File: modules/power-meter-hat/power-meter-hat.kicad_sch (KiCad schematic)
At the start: 25 parts, among them J1 Barrel_Jack_Switch, J2 GPIO, Q1 BC856BDW1, Q2 SI2301CDS, U1 CAT24C256, U2 NCP1117-3.3_SOT223

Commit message: Change jumpers
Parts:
- F1: footprint Fuse:Fuse_1812_4532Metric_Castellated -> Fuse:Fuse_1812_4532Metric

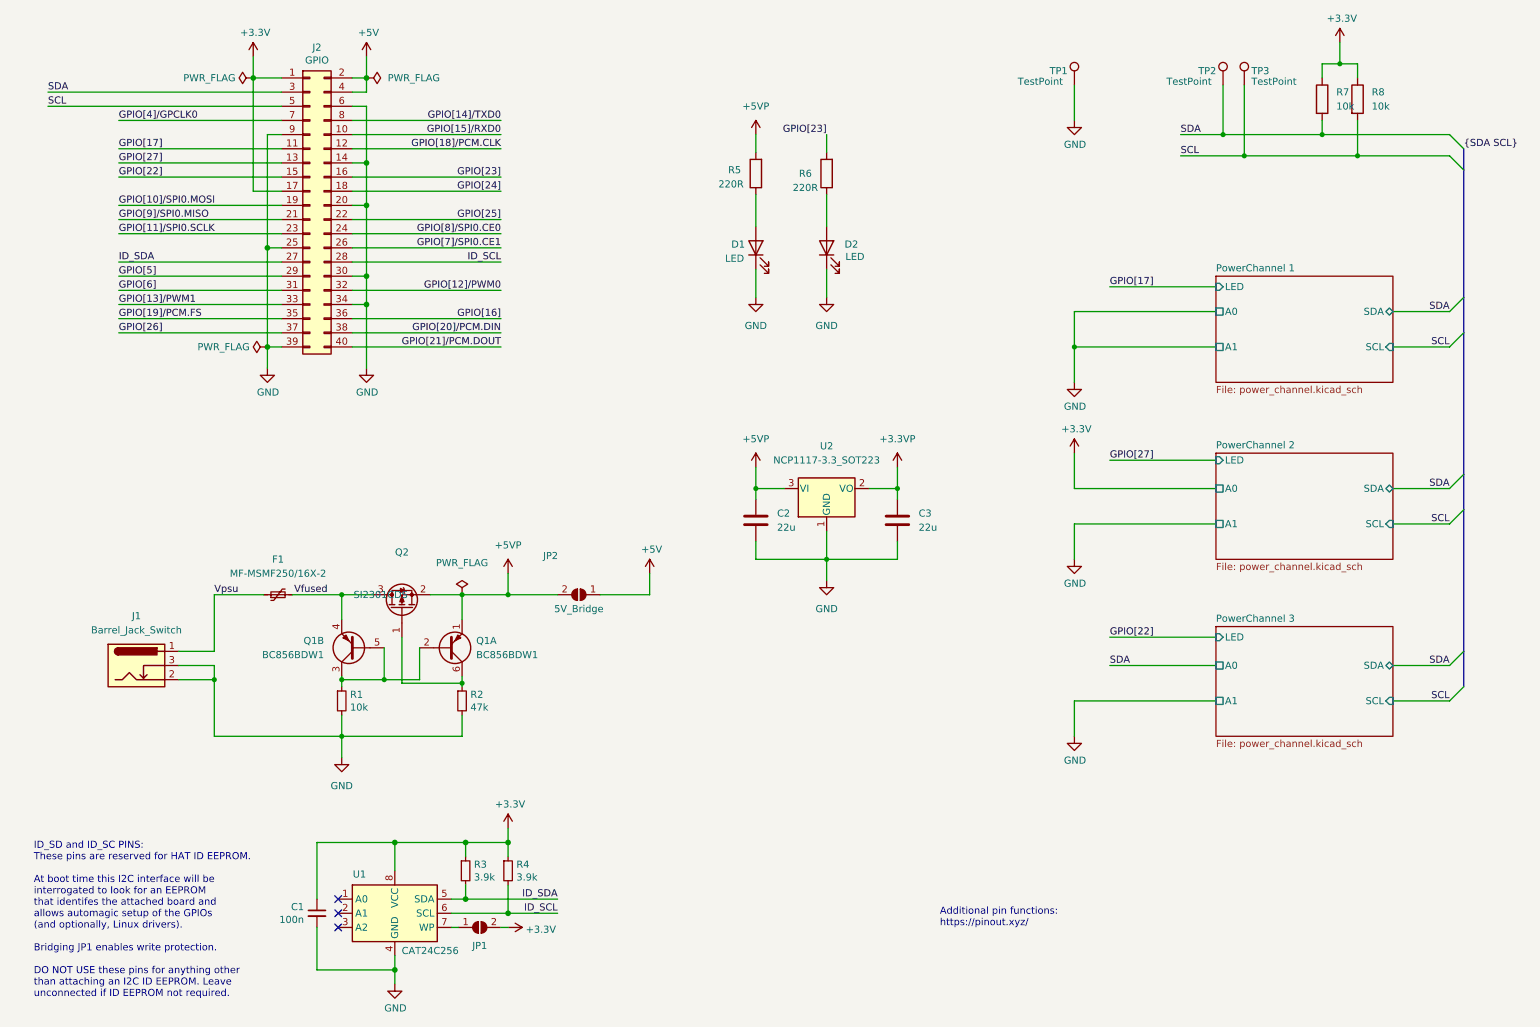
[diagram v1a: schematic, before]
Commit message: Cleanup schematic & PCB
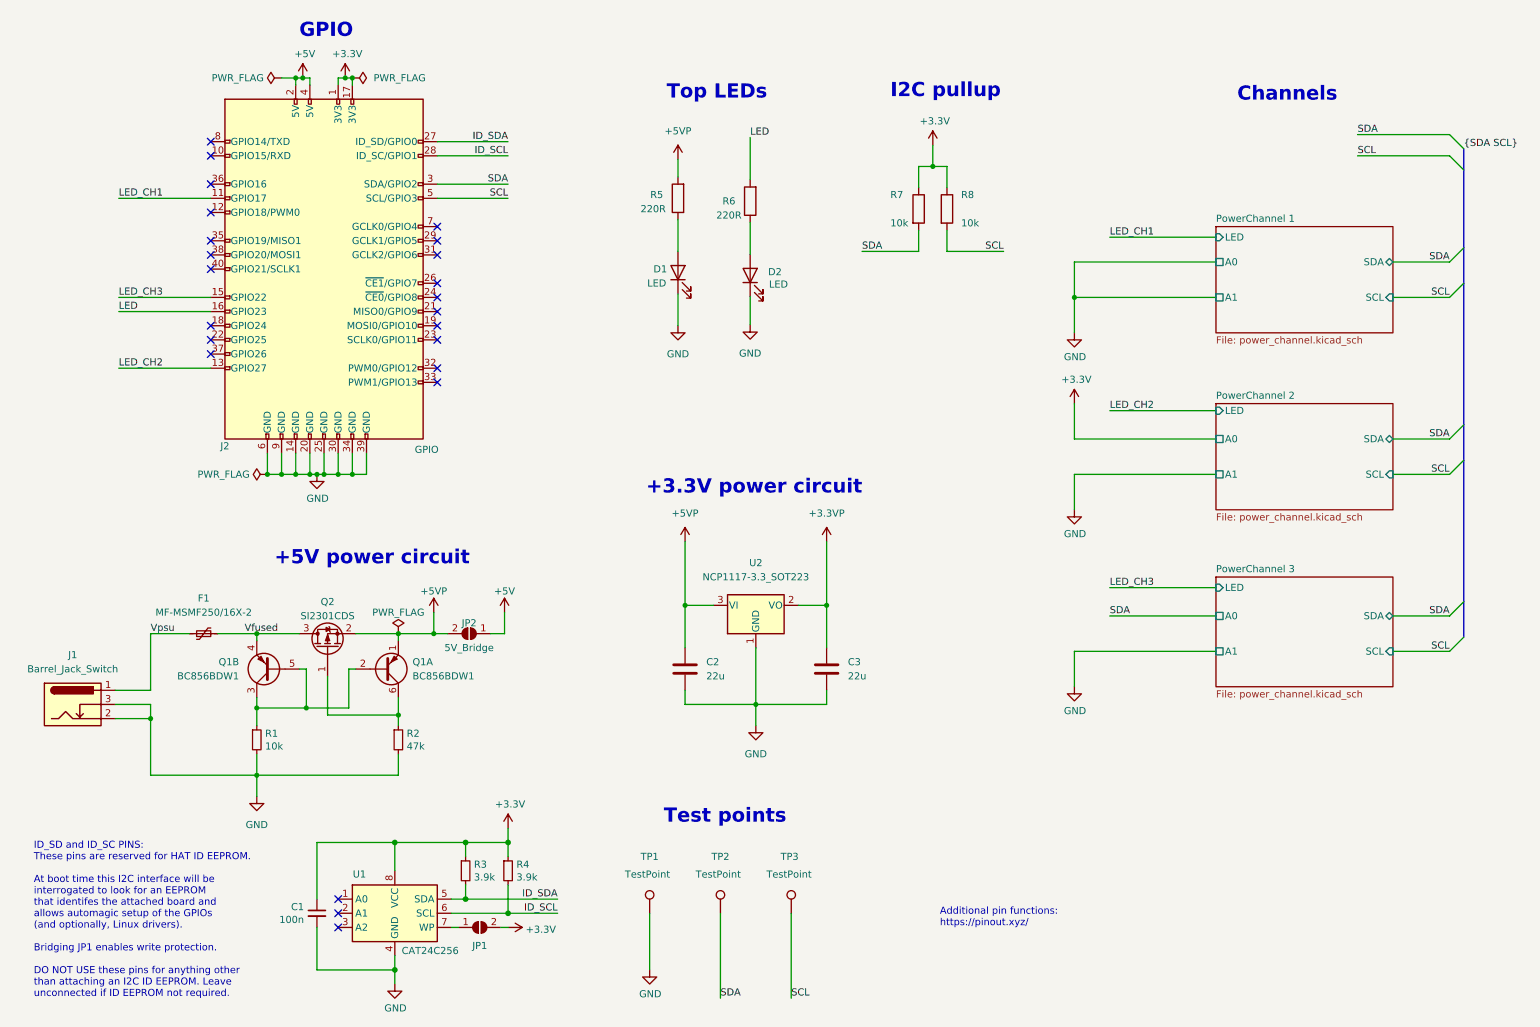
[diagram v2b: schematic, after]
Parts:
- J2: symbol Connector_Generic:Conn_02x20_Odd_Even -> Connector:Raspberry_Pi_2_3
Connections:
- net GPIO[10]/SPI0.MOSI: no longer names the net of J2.19 (MOSI0/GPIO10)
- net GPIO[11]/SPI0.SCLK: no longer names the net of J2.23 (SCLK0/GPIO11)
- net GPIO[12]/PWM0: no longer names the net of J2.32 (PWM0/GPIO12)
- net GPIO[13]/PWM1: no longer names the net of J2.33 (PWM1/GPIO13)
- net GPIO[14]/TXD0: no longer names the net of J2.8 (GPIO14/TXD)
- net GPIO[15]/RXD0: no longer names the net of J2.10 (GPIO15/RXD)
- net GPIO[16]: no longer names the net of J2.36 (GPIO16)
- net GPIO[17] renamed LED_CH1
- net GPIO[18]/PCM.CLK: no longer names the net of J2.12 (GPIO18/PWM0)
- net GPIO[19]/PCM.FS: no longer names the net of J2.35 (GPIO19/MISO1)
- net GPIO[20]/PCM.DIN: no longer names the net of J2.38 (GPIO20/MOSI1)
- net GPIO[21]/PCM.DOUT: no longer names the net of J2.40 (GPIO21/SCLK1)
- net GPIO[22] renamed LED_CH3
- net GPIO[23] renamed LED
- net GPIO[24]: no longer names the net of J2.18 (GPIO24)
- net GPIO[25]: no longer names the net of J2.22 (GPIO25)
- net GPIO[26]: no longer names the net of J2.37 (GPIO26)
- net GPIO[27] renamed LED_CH2
- net GPIO[4]/GPCLK0: no longer names the net of J2.7 (GCLK0/GPIO4)
- net GPIO[5]: no longer names the net of J2.29 (GCLK1/GPIO5)
- net GPIO[6]: no longer names the net of J2.31 (GCLK2/GPIO6)
- net GPIO[7]/SPI0.CE1: no longer names the net of J2.26 (~{CE1}/GPIO7)
- net GPIO[8]/SPI0.CE0: no longer names the net of J2.24 (~{CE0}/GPIO8)
- net GPIO[9]/SPI0.MISO: no longer names the net of J2.21 (MISO0/GPIO9)
- no-connect marks 3 -> 23
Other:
- note added: "+3.3V power circuit"
- note added: "+5V power circuit"
- note added: "Channels"
- note added: "GPIO"
- note added: "I2C pullup"
- note added: "Test points"
- note added: "Top LEDs"
- moved on the sheet: C2, C3, D1, D2, F1, J1, JP2, Q1A, Q1B, Q2, R1, R2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
